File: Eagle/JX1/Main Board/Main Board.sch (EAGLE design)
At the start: 9 parts, among them J1 RASPBERRYPI-40-PIN-GPIO_PTH_N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, U1 SN74HC595N, U2 SN74HC595N

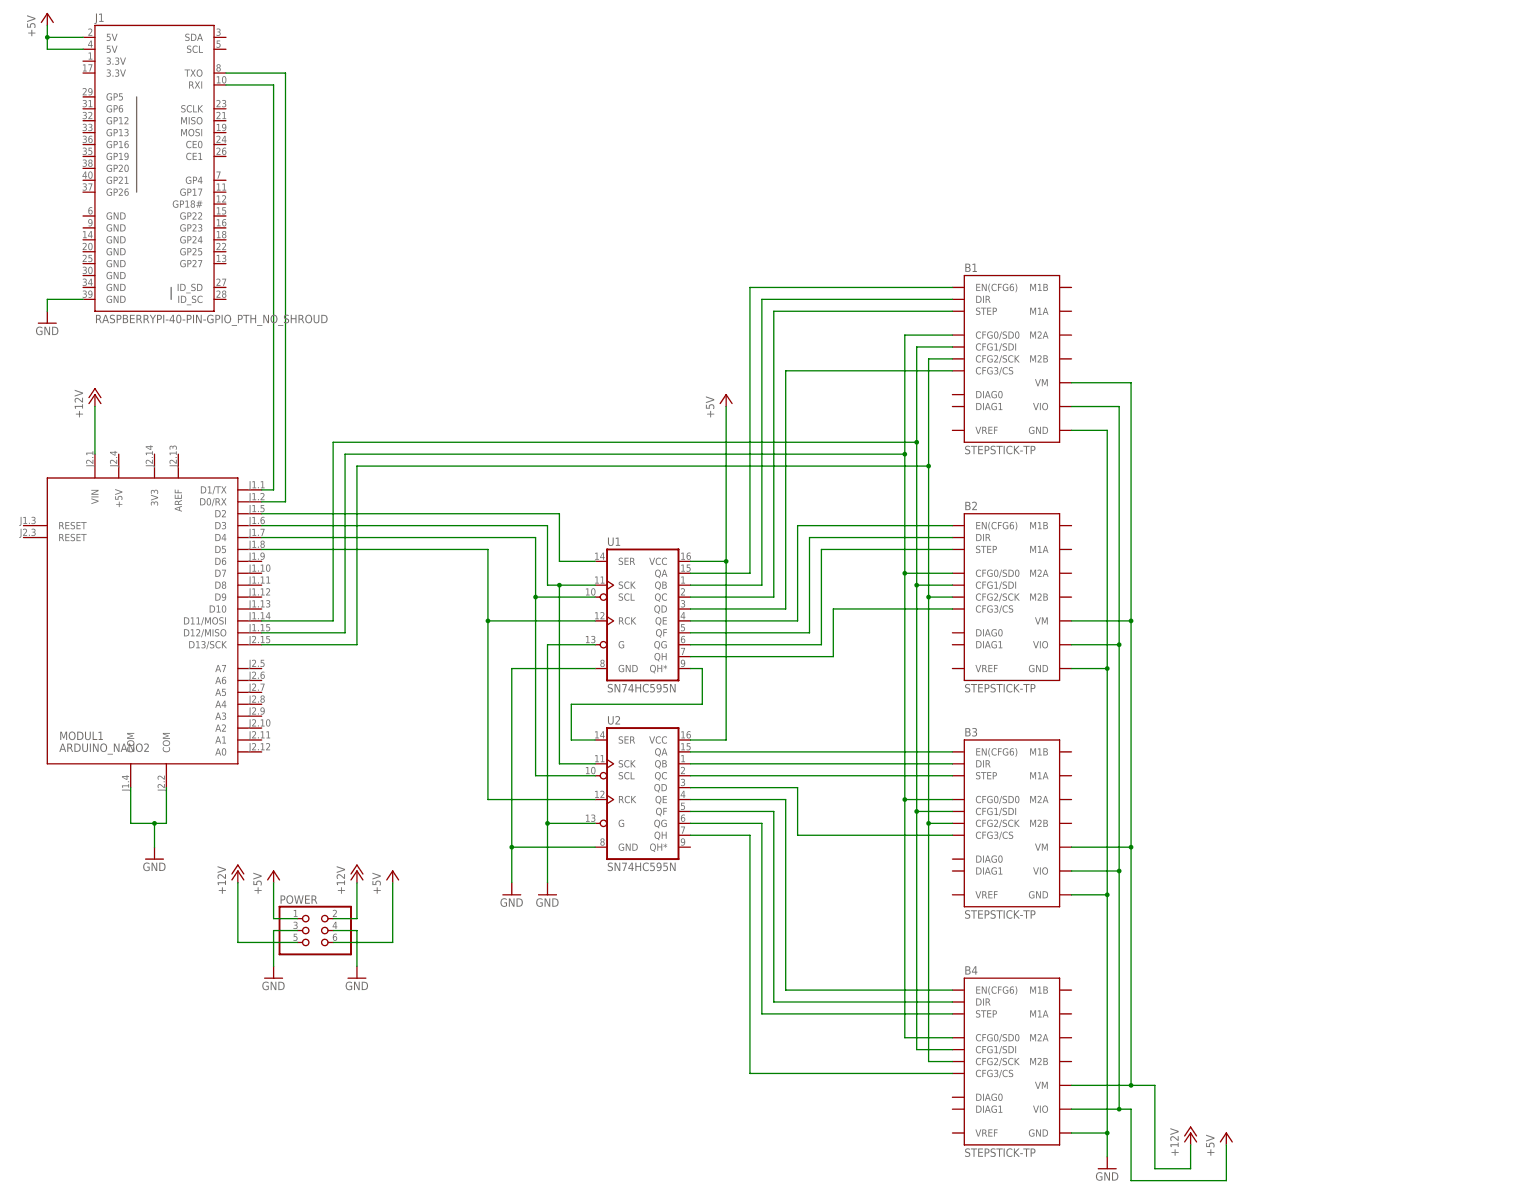
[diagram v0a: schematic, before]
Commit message: More board Changes
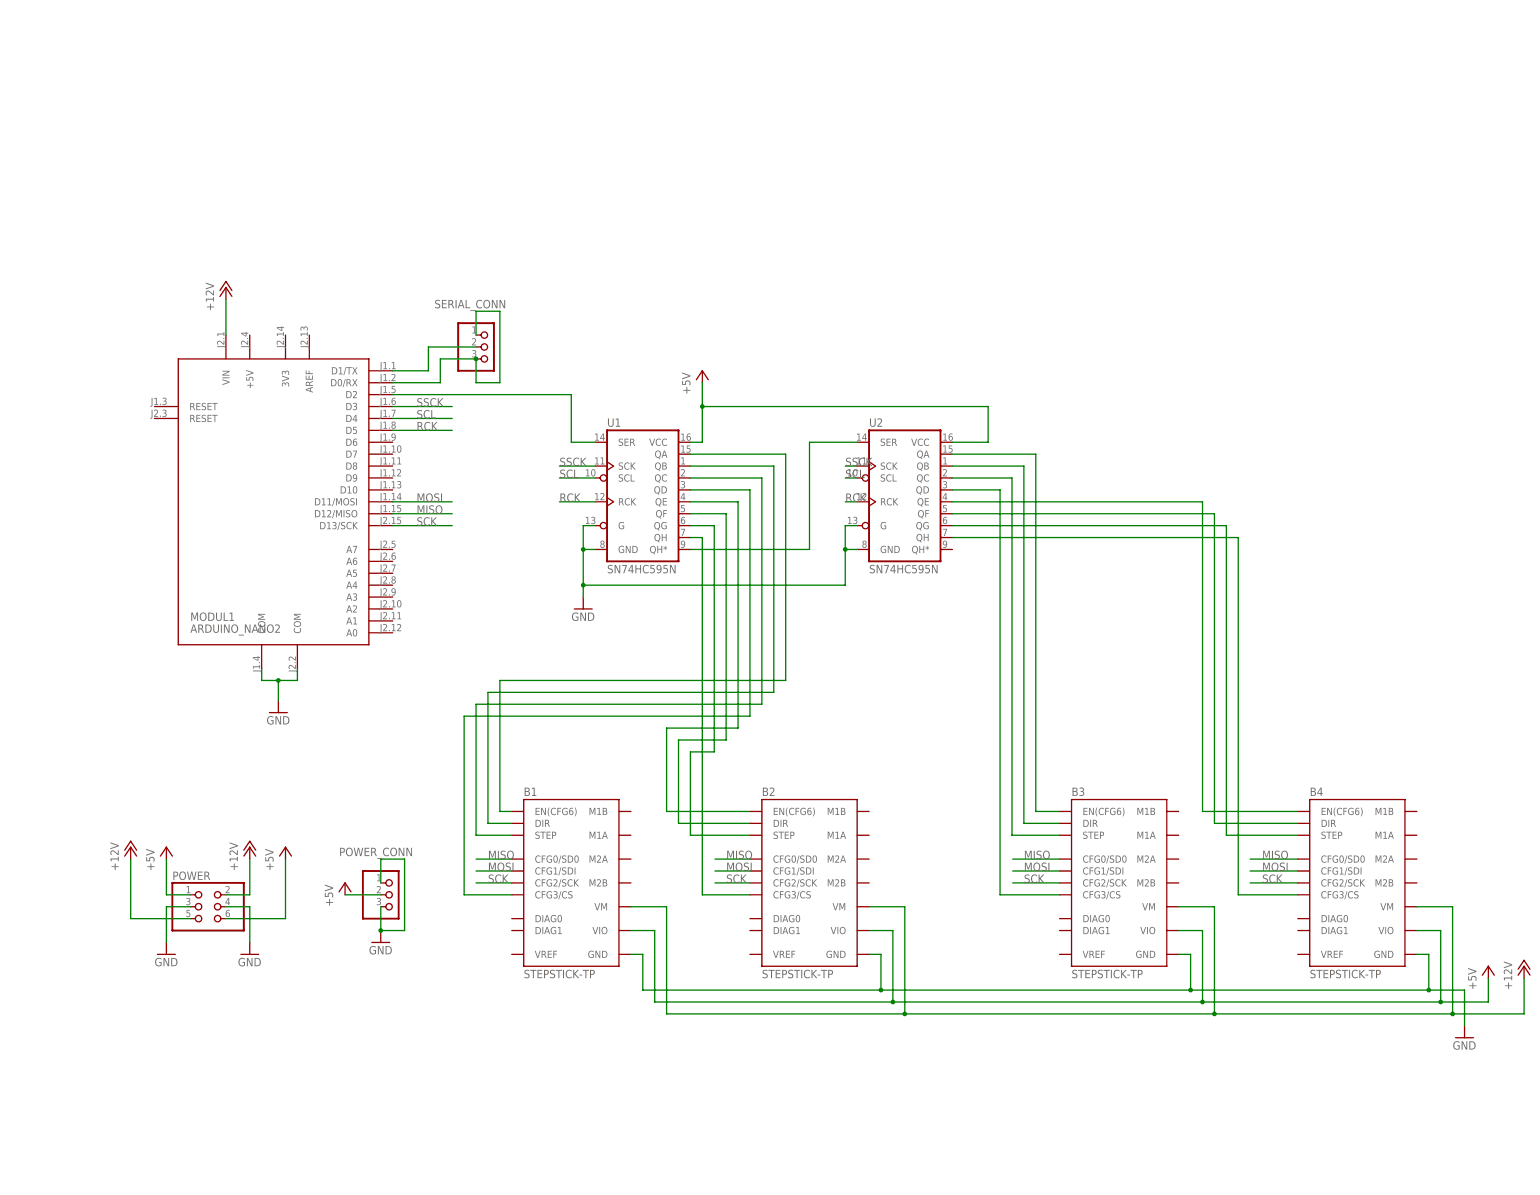
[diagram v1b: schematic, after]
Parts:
- removed J1: RASPBERRYPI-40-PIN-GPIO_PTH_NO_SHROUD, SparkFun-Connectors:RASPBERRYPI-40-PIN-GPIO_PTH_NO_SHROUD
- added POWER_CONN, SERIAL_CONN: (no value), pinhead:PINHD-1X3
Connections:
- net N$19 renamed SCK
- net N$20 renamed MOSI
- net N$21 renamed MISO
- net N$23 renamed SSCK
- net N$24 renamed SCL
- net N$25 renamed RCK
- removed net N$26: J1.RXI, MODUL1.D1/TX
- new net N$1: MODUL1.D1/TX, SERIAL_CONN.2
- net +5V: now also POWER_CONN.2; no longer J1.5V@2, J1.5V@4
- net GND: now also POWER_CONN.1, POWER_CONN.3; no longer J1.GND@39
- net N$27: now also SERIAL_CONN.1, SERIAL_CONN.3; no longer J1.TXO
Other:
- moved on the sheet: B1, B2, B3, B4, MODUL1, POWER, U1, U2
